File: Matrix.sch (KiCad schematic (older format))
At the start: 213 parts

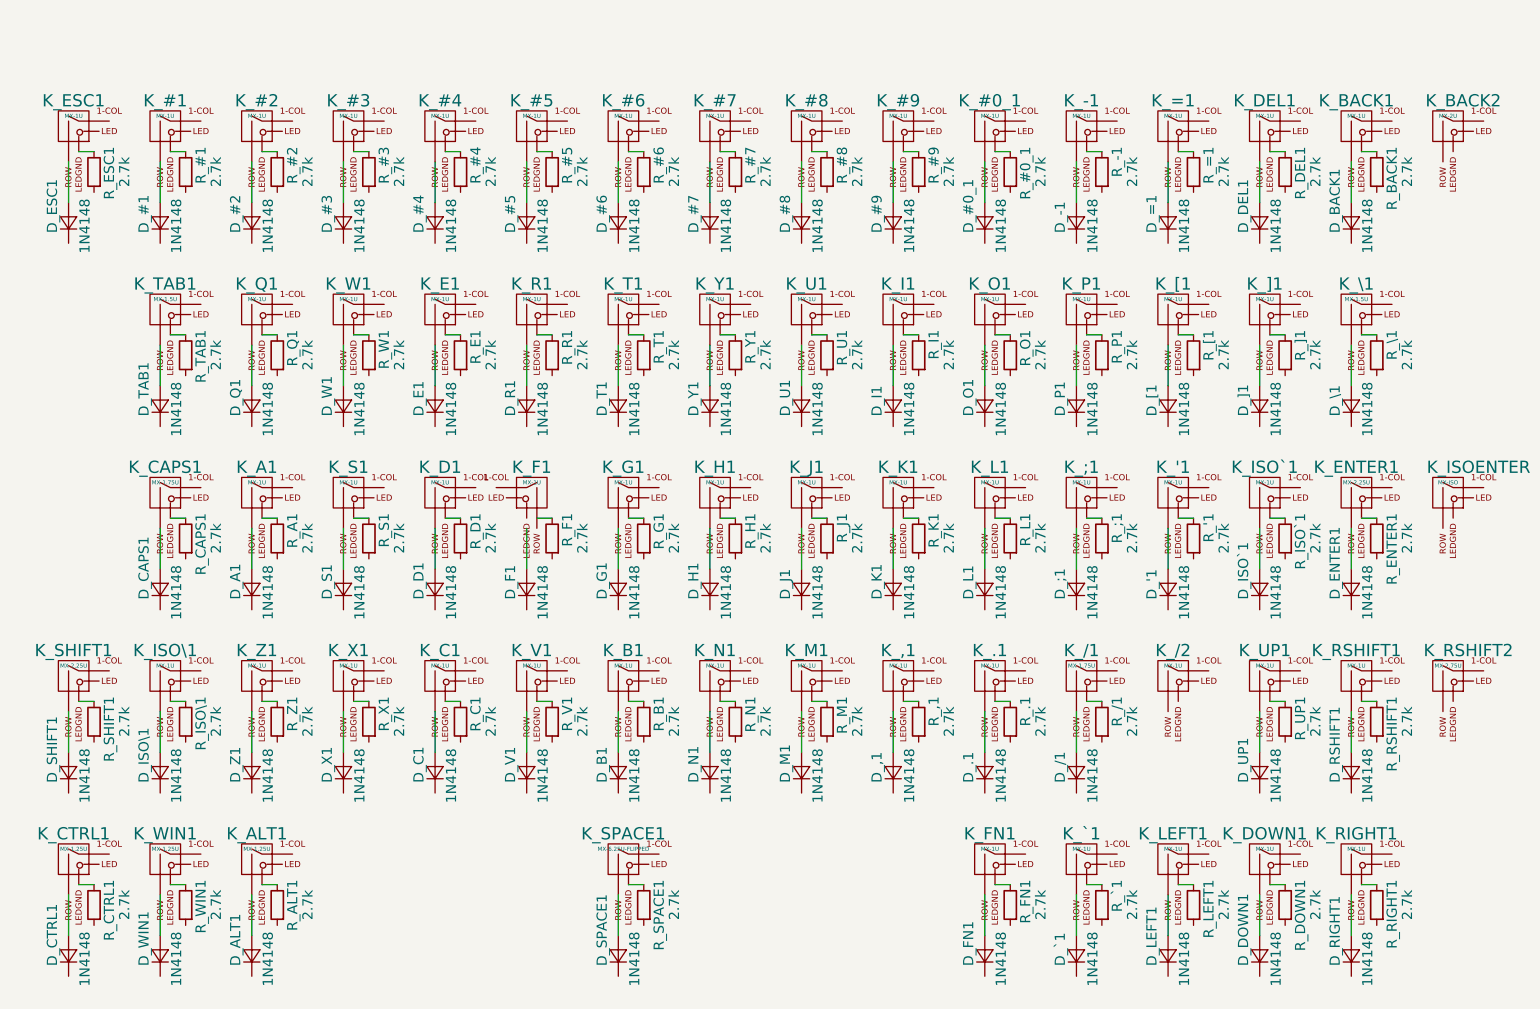
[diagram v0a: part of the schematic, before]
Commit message: Wire cols and 5V rails of LEDs
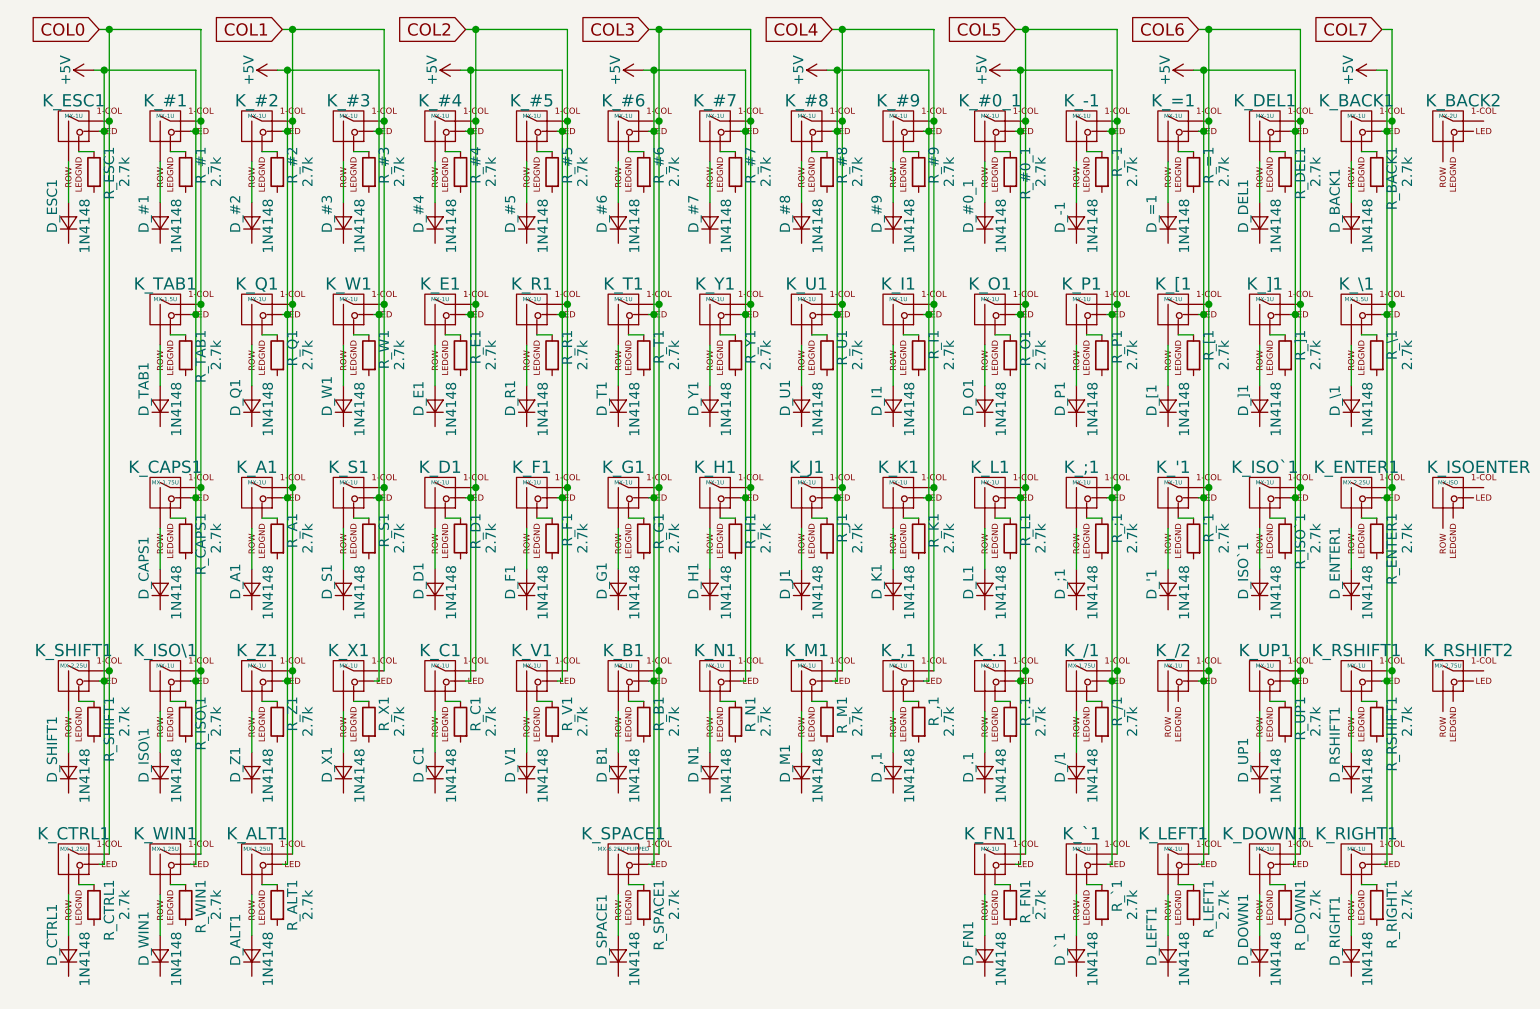
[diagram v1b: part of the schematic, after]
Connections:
- net COL0: now reaches K_ESC1.1 (COL)
- net COL0: now also K_#1.1 (COL), K_CAPS1.1 (COL), K_CTRL1.1 (COL), K_ISO\1.1 (COL), K_SHIFT1.1 (COL), K_TAB1.1 (COL), K_WIN1.1 (COL)
- net +5V: now reaches K_ESC1.3 (LED)
- net +5V: now also K_#0_1.3 (LED), K_#1.3 (LED), K_#2.3 (LED), K_#3.3 (LED), K_#4.3 (LED), K_#5.3 (LED), K_#6.3 (LED), K_#7.3 (LED), K_#8.3 (LED), K_#9.3 (LED), K_'1.3 (LED), K_,1.3 (LED), K_-1.3 (LED), K_.1.3 (LED), K_/1.3 (LED), K_/2.3 (LED), K_;1.3 (LED), K_=1.3 (LED), K_A1.3 (LED), K_ALT1.3 (LED), K_B1.3 (LED), K_BACK1.3 (LED), K_C1.3 (LED), K_CAPS1.3 (LED), K_CTRL1.3 (LED), K_D1.3 (LED), K_DEL1.3 (LED), K_DOWN1.3 (LED), K_E1.3 (LED), K_ENTER1.3 (LED), K_F1.3 (LED), K_FN1.3 (LED), K_G1.3 (LED), K_H1.3 (LED), K_I1.3 (LED), K_ISO\1.3 (LED), K_ISO`1.3 (LED), K_J1.3 (LED), K_K1.3 (LED), K_L1.3 (LED), K_LEFT1.3 (LED), K_M1.3 (LED), K_N1.3 (LED), K_O1.3 (LED), K_P1.3 (LED), K_Q1.3 (LED), K_R1.3 (LED), K_RIGHT1.3 (LED), K_RSHIFT1.3 (LED), K_S1.3 (LED), K_SHIFT1.3 (LED), K_SPACE1.3 (LED), K_T1.3 (LED), K_TAB1.3 (LED), K_U1.3 (LED), K_UP1.3 (LED), K_V1.3 (LED), K_W1.3 (LED), K_WIN1.3 (LED), K_X1.3 (LED), K_Y1.3 (LED), K_Z1.3 (LED), K_[1.3 (LED), K_\1.3 (LED), K_]1.3 (LED), K_`1.3 (LED)
- net COL1: now reaches K_#2.1 (COL)
- net COL1: now also K_#3.1 (COL), K_A1.1 (COL), K_ALT1.1 (COL), K_Q1.1 (COL), K_S1.1 (COL), K_W1.1 (COL), K_X1.1 (COL), K_Z1.1 (COL)
- net COL2: now reaches K_#4.1 (COL)
- net COL2: now also K_#5.1 (COL), K_C1.1 (COL), K_D1.1 (COL), K_E1.1 (COL), K_F1.1 (COL), K_R1.1 (COL), K_V1.1 (COL)
- net COL3: now reaches K_#6.1 (COL)
- net COL3: now also K_#7.1 (COL), K_B1.1 (COL), K_G1.1 (COL), K_H1.1 (COL), K_N1.1 (COL), K_SPACE1.2 (COL), K_T1.1 (COL), K_Y1.1 (COL)
- net COL4: now reaches K_#8.1 (COL)
- net COL4: now also K_#9.1 (COL), K_,1.1 (COL), K_I1.1 (COL), K_J1.1 (COL), K_K1.1 (COL), K_M1.1 (COL), K_U1.1 (COL)
- net COL5: now reaches K_#0_1.1 (COL)
- net COL5: now also K_-1.1 (COL), K_.1.1 (COL), K_/1.1 (COL), K_;1.1 (COL), K_FN1.1 (COL), K_L1.1 (COL), K_O1.1 (COL), K_P1.1 (COL), K_`1.1 (COL)
- net COL6: now reaches K_=1.1 (COL)
- net COL6: now also K_'1.1 (COL), K_/2.1 (COL), K_DEL1.1 (COL), K_DOWN1.1 (COL), K_ISO`1.1 (COL), K_LEFT1.1 (COL), K_UP1.1 (COL), K_[1.1 (COL), K_]1.1 (COL)
- net COL7: now reaches K_BACK1.1 (COL)
- net COL7: now also K_ENTER1.1 (COL), K_RIGHT1.1 (COL), K_RSHIFT1.1 (COL), K_\1.1 (COL)
- net at K_F1.2 (ROW): now also D_F1.2 (A)
- net at K_F1.4 (LEDGND): now also R_F1.2
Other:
- moved on the sheet: K_F1
